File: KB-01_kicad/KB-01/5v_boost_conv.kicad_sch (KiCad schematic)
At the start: 1 part, among them U2 TPS61022

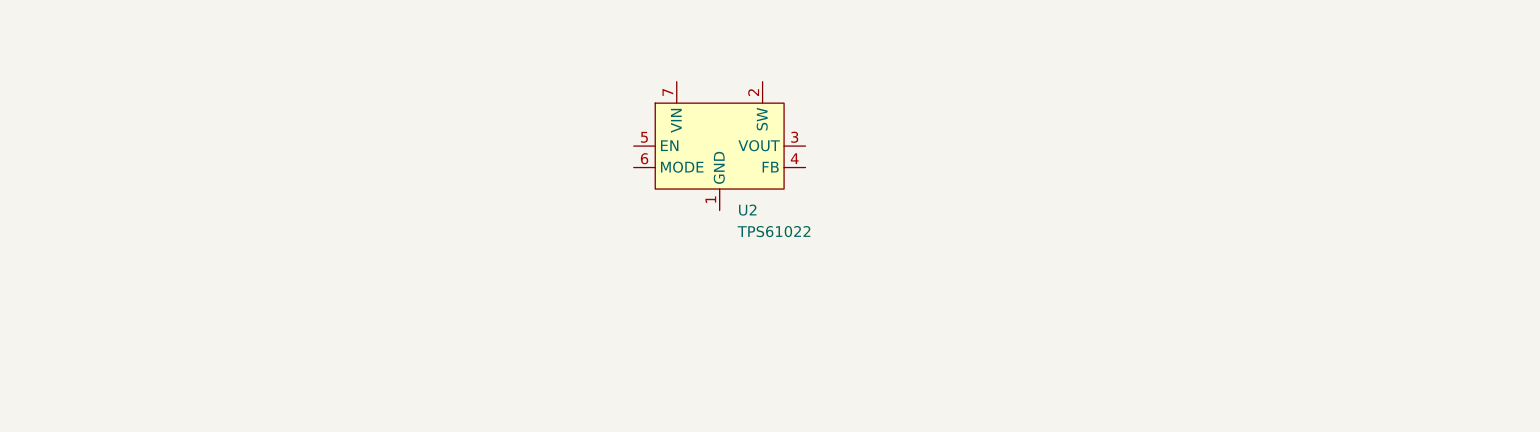
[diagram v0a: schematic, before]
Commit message: all
Signed-off-by: syauqi-alias <syauqi_nur@yahoo.com>
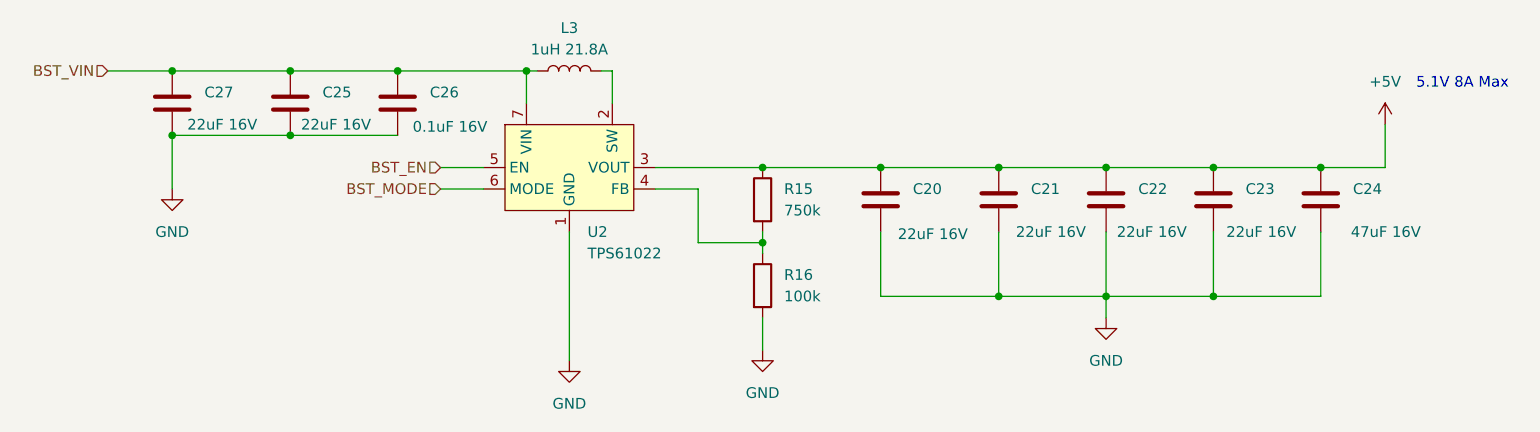
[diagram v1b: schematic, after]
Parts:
- added C20, C21, C22, C23, C25, C27: 22uF 16V, Capacitor_SMD:C_0603_1608Metric_Pad1.08x0.95mm_HandSolder, symbol Device:C
- added C24: 47uF 16V, Capacitor_SMD:C_0603_1608Metric_Pad1.08x0.95mm_HandSolder, symbol Device:C
- added C26: 0.1uF 16V, Capacitor_SMD:C_0603_1608Metric_Pad1.08x0.95mm_HandSolder, symbol Device:C
- added L3: 1uH 21.8A, Inductor_SMD:L_Coilcraft_XAL7030-102, symbol Device:L
- added R15: 750k, Resistor_SMD:R_0603_1608Metric_Pad0.98x0.95mm_HandSolder, symbol Device:R
- added R16: 100k, Resistor_SMD:R_0603_1608Metric_Pad0.98x0.95mm_HandSolder, symbol Device:R
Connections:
- net GND: now reaches U2.1 (GND)
- net GND: now also C20.2, C21.2, C22.2, C23.2, C24.2, C25.2, C26.2, C27.2, R16.2
- net at U2.2 (SW): now also L3.2
- net +5V: now reaches U2.3 (VOUT)
- net +5V: now also C20.1, C21.1, C22.1, C23.1, C24.1, R15.1
- net at U2.4 (FB): now also R15.2, R16.1
- net BST_EN: now reaches U2.5 (EN)
- net BST_MODE: now reaches U2.6 (MODE)
- net BST_VIN: now reaches U2.7 (VIN)
- net BST_VIN: now also C25.1, C26.1, C27.1, L3.1
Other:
- note added: "5.1V 8A Max"
- moved on the sheet: U2
